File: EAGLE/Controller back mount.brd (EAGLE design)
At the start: 40.6 x 27.9 mm, 47 parts, among them IC1 TPS77033, IC2 TPS77033, J2 USB-MICROB, T3 MMBT3906LT1SMD, U1 ATMEGA328P_TQFP, U2 MCP73831, Y1 16MHz

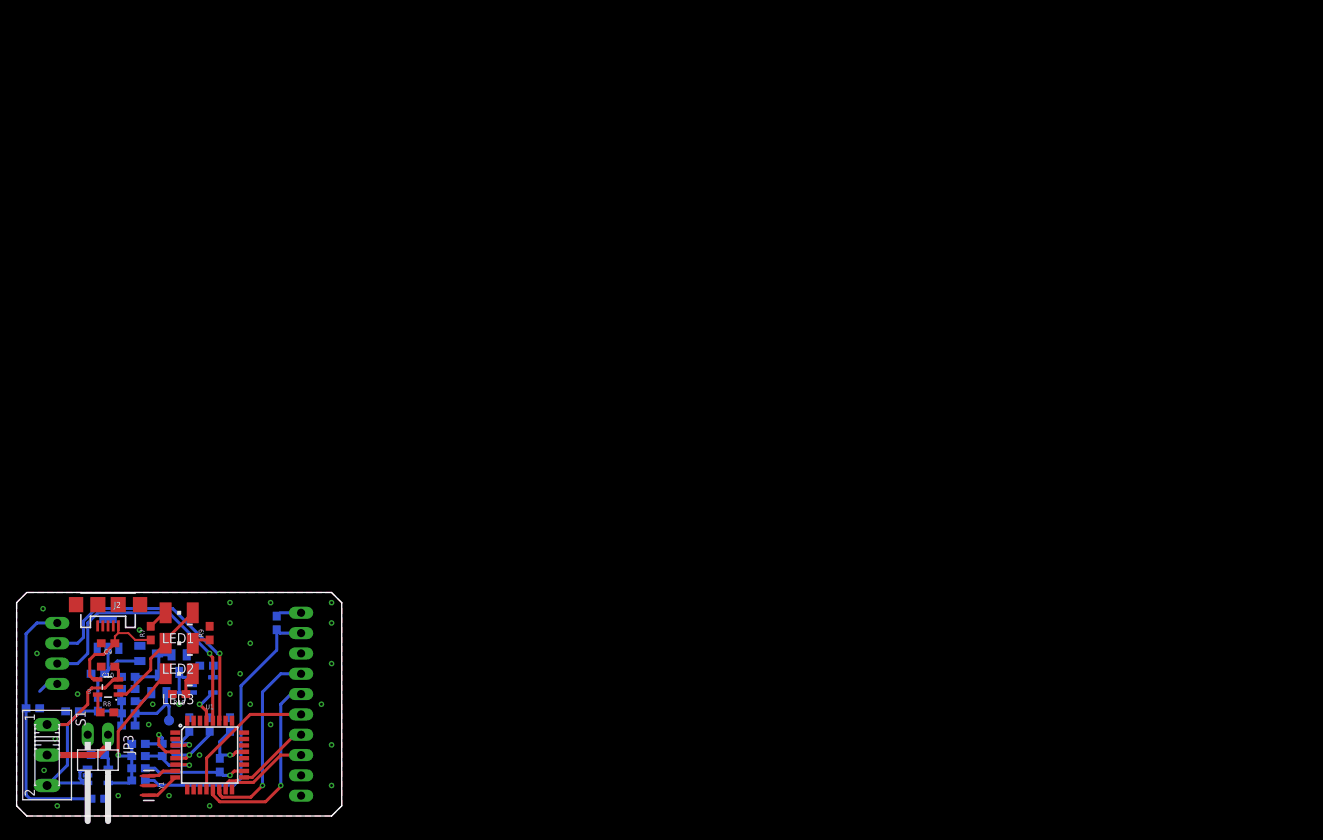
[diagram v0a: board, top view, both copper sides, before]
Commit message: Prototype Structure
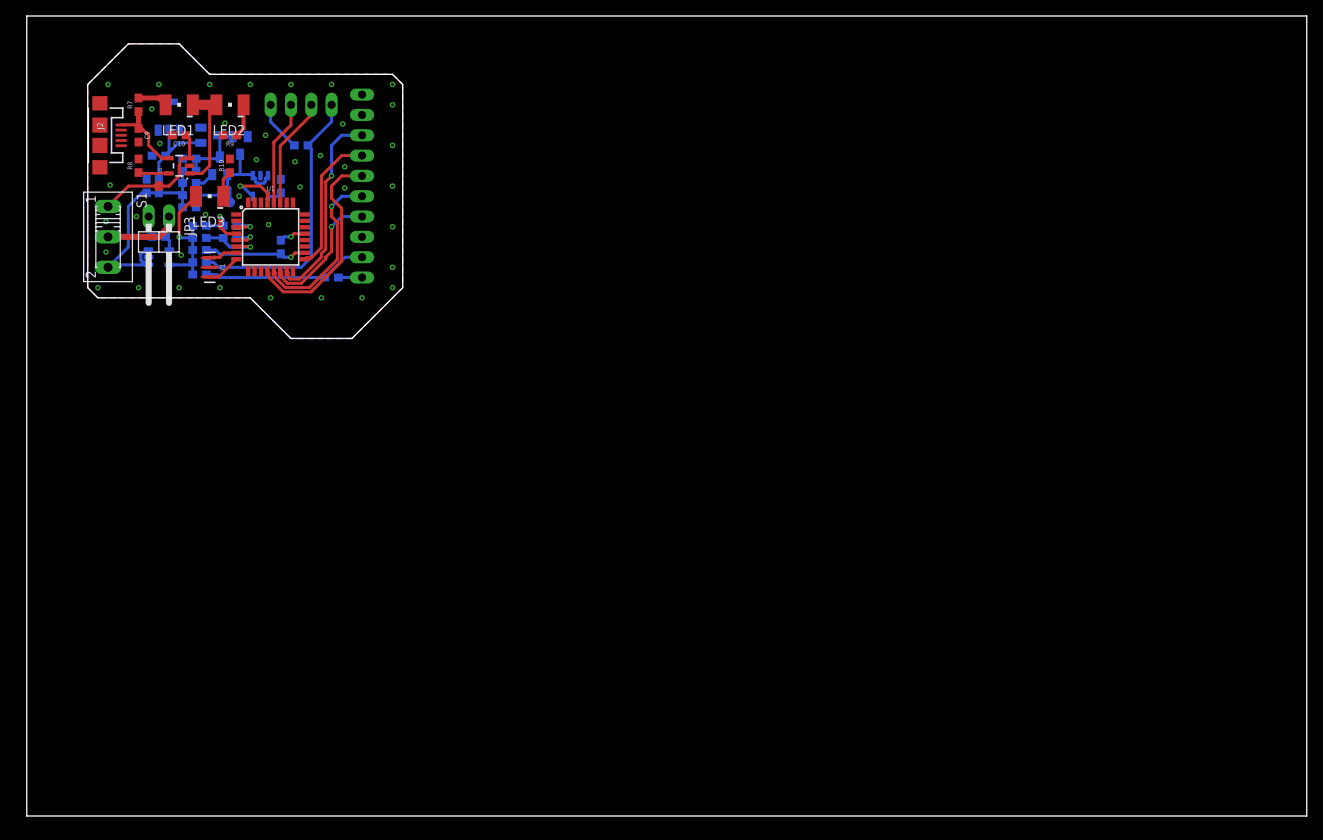
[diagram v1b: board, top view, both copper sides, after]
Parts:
- removed R12, R13, R4: 0, SparkFun-Resistors:0603
- added TP2: TEST-POINT3X5, SparkFun-Connectors:PAD.03X.05
- JP2: device pinhead:1X04/90 -> pinhead:1X04
- moved C11 77.9 mm to (34.3, 83.8), turned to 0 degrees
- moved JP2 76.7 mm to (34.3, 88.9), turned to 0 degrees
- moved R8 68.4 mm to (14.0, 81.3), turned to 90 degrees
- moved FB4 68.2 mm to (21.6, 69.2), turned to 180 degrees
- moved LED2 67.6 mm to (25.4, 88.9)
- moved C10 67.0 mm to (19.1, 85.1)
- moved R10 66.3 mm to (25.4, 81.3), turned to 90 degrees
- moved C7 66.3 mm to (15.0, 78.7), turned to 90 degrees
- moved R7 66.1 mm to (14.0, 88.9)
- moved U2 65.8 mm to (19.1, 81.3)
- moved C1 65.2 mm to (31.8, 71.1)
- moved C2 65.2 mm to (25.4, 73.8)
- moved C3 65.2 mm to (25.4, 72.3)
- moved FB1 65.2 mm to (21.6, 70.7)
- moved FB2 65.2 mm to (21.6, 73.8)
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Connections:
- new net CAM_GND: C11.2, JP2.4
- new net OLED_GND: C12.2, JP1.1
- net AGND: no longer R13.2
- net GND: no longer C11.2, C12.2, JP1.10, JP2.4, R12.1, R13.1, R4.1
- net GND1: no longer R12.2
- net GND2: no longer R4.2
- net N$13: now also TP2.P$1
- net OLED_DC: now also JP1.6; no longer JP1.5
- net OLED_MOSI: now also JP1.8; no longer JP1.3
- net OLED_OC: now also JP1.4; no longer JP1.7
- net OLED_RESET: now also JP1.5; no longer JP1.6
- net OLED_SCK: now also JP1.7; no longer JP1.4
- net OLED_VCC: now also JP1.2; no longer JP1.9
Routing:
- net CAM_SCL: track 34.6 -> 13.1 mm, vias 1 -> 0
- net CAM_SDA: track 34.1 -> 13.8 mm, vias 1 -> 0
- net OLED_VCC: track 36.3 -> 20.7 mm
- net OLED_MOSI: track 11.7 -> 25.1 mm, vias 0 -> 1
- net OLED_DC: track 18.0 -> 26.5 mm
- net OLED_SCK: track 9.35 -> 17.8 mm
- net OLED_OC: track 24.2 -> 16.6 mm
- net N$8: track 23.8 -> 16.9 mm
- net CAM_GND: track 0.00 -> 6.31 mm
- net GND: track 5.21 -> 0.00 mm, vias 28 -> 39
- net GND2: track 7.85 -> 3.66 mm
- net AGND: track 7.09 -> 3.36 mm
- net N$11: track 14.0 -> 10.7 mm
- net OLED_GND: track 0.00 -> 2.96 mm
- net N$13: track 13.9 -> 16.8 mm
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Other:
- board size 40.6 x 27.9 mm -> 160 x 100 mm
